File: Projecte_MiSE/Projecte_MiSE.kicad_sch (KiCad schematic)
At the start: 45 parts, among them IC1 MSP430FR2355TPT, J1 C_DFrobot, J10 Conn_GND_TP, J11 Conn_TXD_TP, J12 Conn_RXD_TP, J2 Conn_SWB, J3 ESP01_WIFI, J4 URM10, J5 Conn_GND_TP, J6 Conn_ACLK_TP, J7 Conn_SMCLK_TP, J8 Conn_SDA_TP, J9 Conn_SCL_TP, SW1 ~{RST}, U1 LMV324, Y1 Crystal_GND3

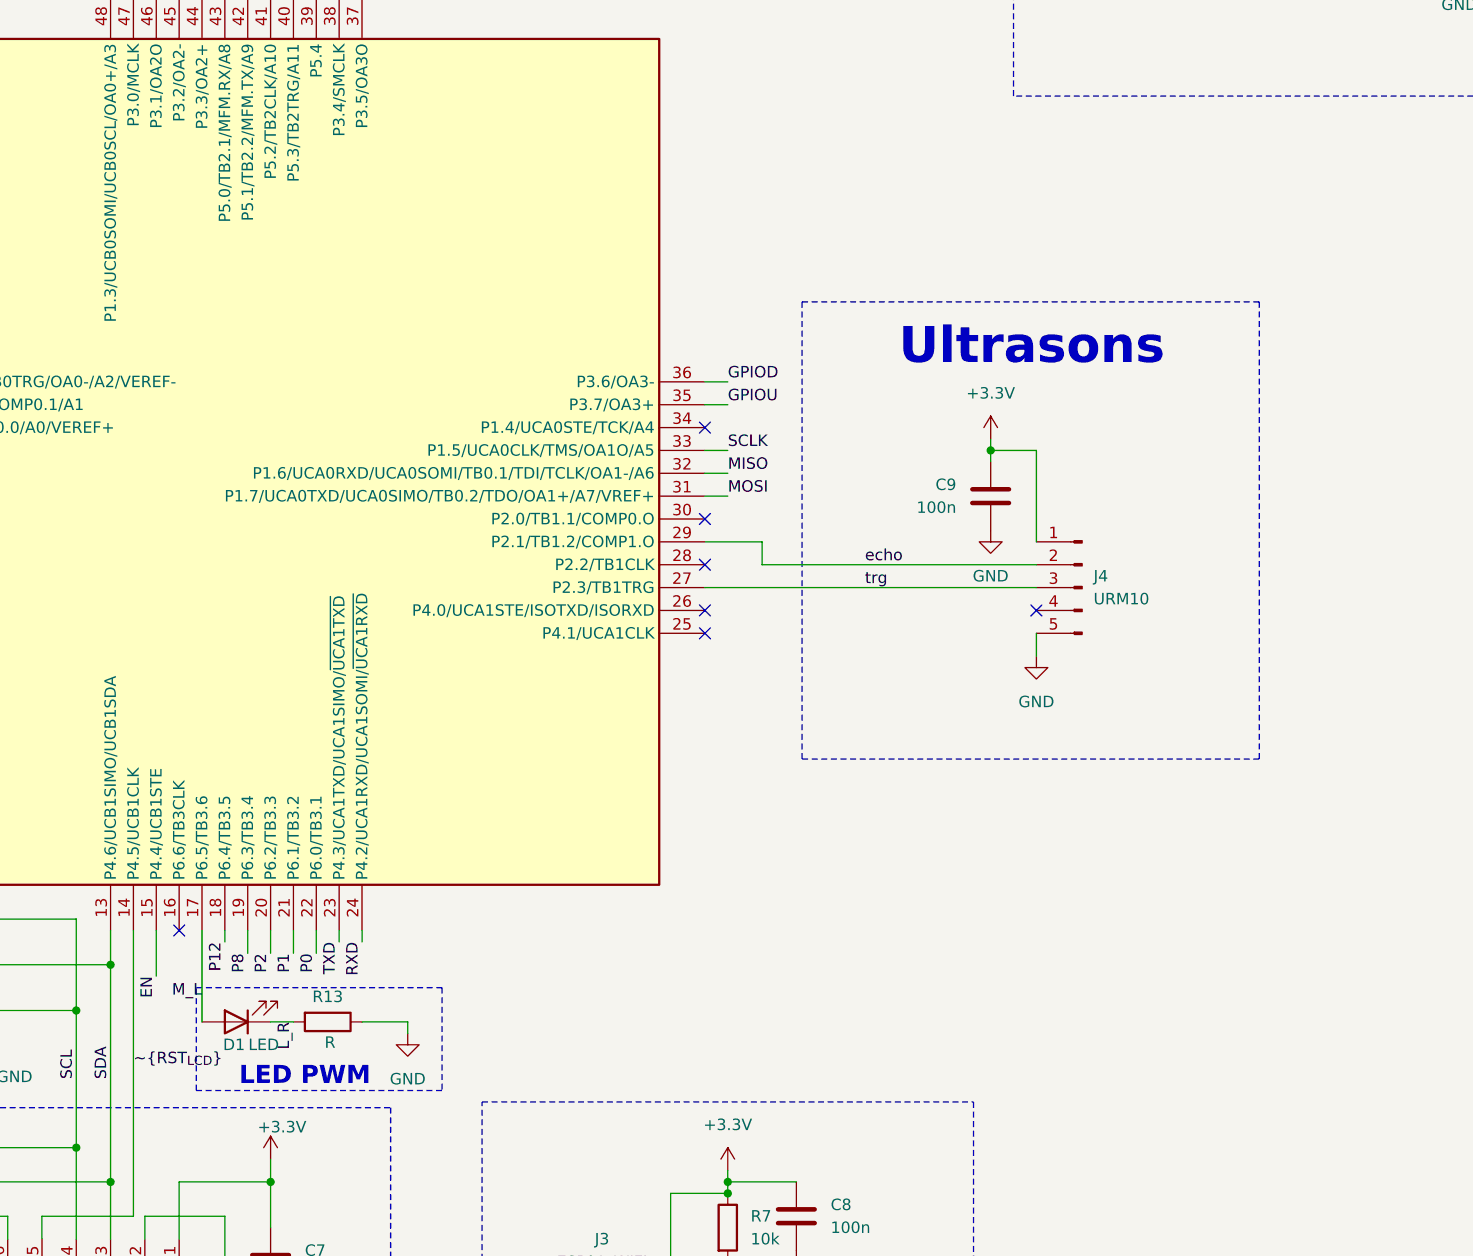
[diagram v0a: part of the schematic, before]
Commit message: footprints and layout
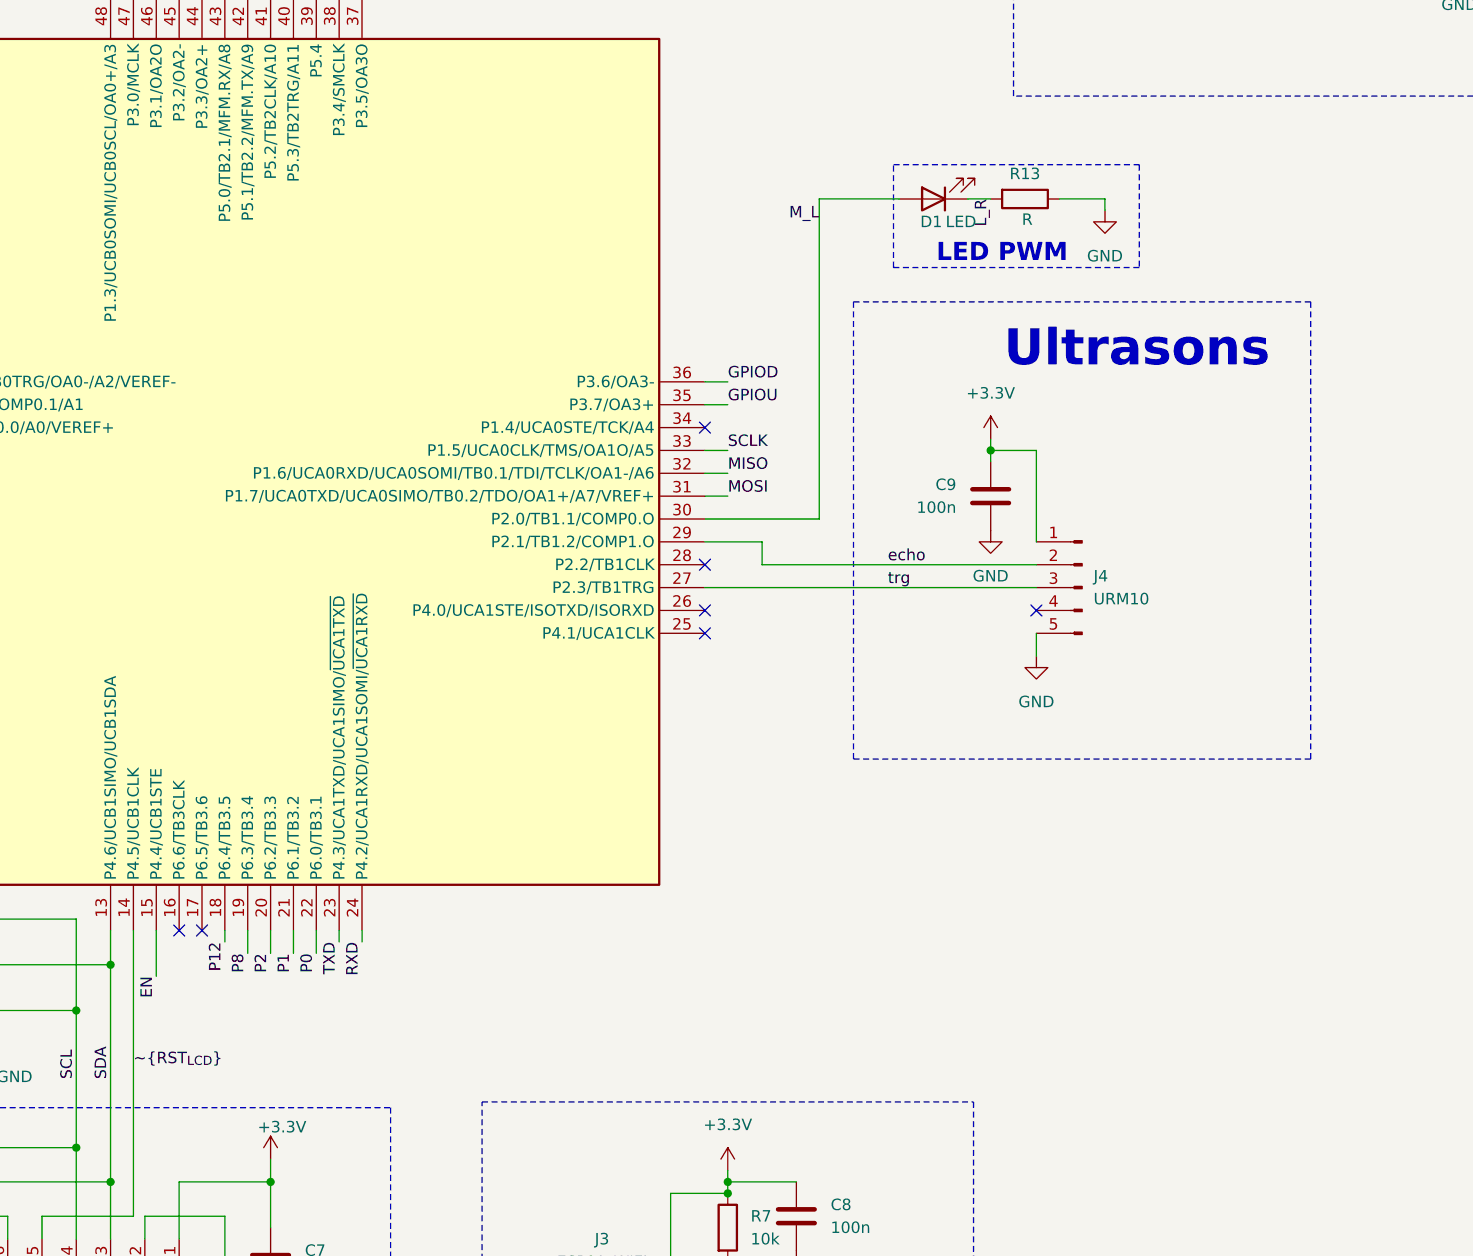
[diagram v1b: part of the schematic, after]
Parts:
- J10, J11, J12, J5, J6, J7, J8, J9: footprint Connector_PinHeader_1.00mm:PinHeader_1x01_P1.00mm_Vertical -> Connector_PinHeader_2.54mm:PinHeader_1x01_P2.54mm_Vertical
- J4: footprint Connector_PinSocket_2.54mm:PinSocket_1x05_P2.54mm_Vertical -> Connector_PinHeader_2.54mm:PinHeader_1x05_P2.54mm_Vertical
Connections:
- net M_L: now also IC1.30 (P2.0/TB1.1/COMP0.O); no longer IC1.17 (P6.5/TB3.6)
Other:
- moved on the sheet: D1, R13
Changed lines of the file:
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@@
 	)
 	(rectangle
-		(start 159.385 215.9)
-		(end 186.69 227.33)
+		(start 236.855 124.46)
+		(end 264.16 135.89)
 		(stroke
 			(width 0)
@@
 	)
 	(rectangle
-		(start 226.695 139.7)
-		(end 277.495 190.5)
+		(start 232.41 139.7)
+		(end 283.21 190.5)
 		(stroke
 			(width 0)
@@
 	(text "Ultrasons\n"
 		(exclude_from_sim no)
-		(at 252.222 144.78 0)
+		(at 263.906 145.034 0)
 		(effects
 			(font
@@
 	(text "LED PWM"
 		(exclude_from_sim no)
-		(at 171.45 225.806 0)
+		(at 248.92 134.366 0)
 		(effects
 			(font
@@
 	)
 	(no_connect
-		(at 215.9 163.83)
-	)
-	(no_connect
 		(at 252.73 173.99)
 	)
@@
 	)
 	(no_connect
+		(at 160.02 209.55)
+	)
+	(no_connect
 		(at 210.82 252.73)
 	)
@@
 	(wire
 		(pts
+			(xy 215.9 163.83) (xy 228.6 163.83)
+		)
+		(stroke
+			(width 0)
+			(type default)
+		)
+	)
+	(wire
+		(pts
 			(xy 66.04 247.65) (xy 69.85 247.65)
 		)
@@
 	(wire
 		(pts
+			(xy 228.6 128.27) (xy 237.49 128.27)
+		)
+		(stroke
+			(width 0)
+			(type default)
+		)
+	)
+	(wire
+		(pts
 			(xy 49.53 149.86) (xy 49.53 151.13)
 		)
@@
 	(wire
 		(pts
+			(xy 228.6 163.83) (xy 228.6 128.27)
+		)
+		(stroke
+			(width 0)
+			(type default)
+		)
+	)
+	(wire
+		(pts
 			(xy 187.96 68.58) (xy 187.96 71.12)
 		)
@@
 	(wire
 		(pts
-			(xy 160.02 209.55) (xy 160.02 219.71)
-		)
-		(stroke
-			(width 0)
-			(type default)
-		)
-	)
-	(wire
-		(pts
 			(xy 317.5 91.44) (xy 317.5 99.06)
 		)
@@
 	(wire
 		(pts
-			(xy 177.8 219.71) (xy 182.88 219.71)
+			(xy 255.27 128.27) (xy 260.35 128.27)
 		)
 		(stroke
@@
 	(wire
 		(pts
-			(xy 167.64 219.71) (xy 170.18 219.71)
+			(xy 245.11 128.27) (xy 247.65 128.27)
 		)
 		(stroke
@@
 	(wire
 		(pts
-			(xy 182.88 219.71) (xy 182.88 220.98)
+			(xy 260.35 128.27) (xy 260.35 129.54)
 		)
 		(stroke
@@
 	)
 	(label "M_L"
-		(at 160.02 217.17 180)
+		(at 228.6 130.81 180)
 		(effects
 			(font
@@
 	)
 	(label "echo"
-		(at 233.68 168.91 0)
+		(at 236.22 168.91 0)
 		(effects
 			(font
@@
 	)
 	(label "trg"
-		(at 233.68 171.45 0)
+		(at 236.22 171.45 0)
 		(effects
 			(font
@@
 	)
 	(label "L_R"
-		(at 170.18 219.71 270)
+		(at 247.65 128.27 270)
 		(effects
 			(font
@@
 			)
 		)
-		(property "Footprint" "Connector_PinHeader_1.00mm:PinHeader_1x01_P1.00mm_Vertical"
+		(property "Footprint" "Connector_PinHeader_2.54mm:PinHeader_1x01_P2.54mm_Vertical"
 			(at 128.27 213.36 0)
 			(effects
@@
 	(symbol
 		(lib_id "power:GND")
-		(at 182.88 220.98 0)
+		(at 260.35 129.54 0)
 		(unit 1)
 		(exclude_from_sim no)
@@
 		(fields_autoplaced yes)
 		(property "Reference" "#PWR025"
-			(at 182.88 227.33 0)
+			(at 260.35 135.89 0)
 			(effects
 				(font
@@
 		)
 		(property "Value" "GND"
-			(at 182.88 226.06 0)
+			(at 260.35 134.62 0)
 			(effects
 				(font
@@
 		)
 		(property "Footprint" ""
-			(at 182.88 220.98 0)
+			(at 260.35 129.54 0)
 			(effects
 				(font
@@
 		)
 		(property "Datasheet" ""
-			(at 182.88 220.98 0)
+			(at 260.35 129.54 0)
 			(effects
 				(font
@@
 		)
 		(property "Description" "Power symbol creates a global label with name \"GND\" , ground"
-			(at 182.88 220.98 0)
+			(at 260.35 129.54 0)
 			(effects
 				(font
@@
 			)
 		)
-		(property "Footprint" "Connector_PinHeader_1.00mm:PinHeader_1x01_P1.00mm_Vertical"
+		(property "Footprint" "Connector_PinHeader_2.54mm:PinHeader_1x01_P2.54mm_Vertical"
 			(at 231.14 252.73 0)
 			(effects
@@
 	(symbol
 		(lib_id "Device:R")
-		(at 173.99 219.71 270)
+		(at 251.46 128.27 270)
 		(unit 1)
 		(exclude_from_sim no)
@@
 		(dnp no)
 		(property "Reference" "R13"
-			(at 173.99 216.916 90)
+			(at 251.46 125.476 90)
 			(effects
 				(font
@@
 		)
 		(property "Value" "R"
-			(at 174.244 221.996 90)
+			(at 251.714 130.556 90)
 			(effects
 				(font
@@
 		)
 		(property "Footprint" "Resistor_SMD:R_0805_2012Metric"
-			(at 173.99 217.932 90)
+			(at 251.46 126.492 90)
 			(effects
 				(font
@@
 		)
 		(property "Datasheet" "~"
-			(at 173.99 219.71 0)
+			(at 251.46 128.27 0)
 			(effects
 				(font
@@
 		)
 		(property "Description" "Resistor"
-			(at 173.99 219.71 0)
+			(at 251.46 128.27 0)
 			(effects
 				(font
@@
 			)
 		)
-		(property "Footprint" "Connector_PinHeader_1.00mm:PinHeader_1x01_P1.00mm_Vertical"
+		(property "Footprint" "Connector_PinHeader_2.54mm:PinHeader_1x01_P2.54mm_Vertical"
 			(at 76.2 105.41 0)
 			(effects
@@
 			)
 		)
-		(property "Footprint" "Connector_PinHeader_1.00mm:PinHeader_1x01_P1.00mm_Vertical"
+		(property "Footprint" "Connector_PinHeader_2.54mm:PinHeader_1x01_P2.54mm_Vertical"
 			(at 74.93 111.76 0)
 			(effects
@@
 			)
 		)
-		(property "Footprint" "Connector_PinHeader_1.00mm:PinHeader_1x01_P1.00mm_Vertical"
+		(property "Footprint" "Connector_PinHeader_2.54mm:PinHeader_1x01_P2.54mm_Vertical"
 			(at 128.27 218.44 0)
 			(effects
@@
 			)
 		)
-		(property "Footprint" "Connector_PinHeader_1.00mm:PinHeader_1x01_P1.00mm_Vertical"
+		(property "Footprint" "Connector_PinHeader_2.54mm:PinHeader_1x01_P2.54mm_Vertical"
 			(at 128.27 224.79 0)
 			(effects
@@
 			)
 		)
-		(property "Footprint" "Connector_PinHeader_1.00mm:PinHeader_1x01_P1.00mm_Vertical"
+		(property "Footprint" "Connector_PinHeader_2.54mm:PinHeader_1x01_P2.54mm_Vertical"
 			(at 76.2 100.33 0)
 			(effects
@@
 			)
 		)
-		(property "Footprint" "Connector_PinHeader_1.00mm:PinHeader_1x01_P1.00mm_Vertical"
+		(property "Footprint" "Connector_PinHeader_2.54mm:PinHeader_1x01_P2.54mm_Vertical"
 			(at 229.87 257.81 0)
 			(effects
@@
 	(symbol
 		(lib_id "Device:LED")
-		(at 163.83 219.71 180)
+		(at 241.3 128.27 180)
 		(unit 1)
 		(exclude_from_sim no)
@@
 		(dnp no)
 		(property "Reference" "D1"
-			(at 163.576 222.25 0)
+			(at 241.046 130.81 0)
 			(effects
 				(font
@@
 		)
 		(property "Value" "LED"
-			(at 166.878 222.25 0)
+			(at 244.348 130.81 0)
 			(effects
 				(font
@@
 		)
 		(property "Footprint" "LED_SMD:LED_0805_2012Metric"
-			(at 163.83 219.71 0)
+			(at 241.3 128.27 0)
 			(effects
 				(font
@@
 		)
 		(property "Datasheet" "~"
-			(at 163.83 219.71 0)
+			(at 241.3 128.27 0)
 			(effects
 				(font
@@
 		)
 		(property "Description" "Light emitting diode"
-			(at 163.83 219.71 0)
+			(at 241.3 128.27 0)
 			(effects
 				(font
@@
 			)
 		)
-		(property "Footprint" "Connector_PinSocket_2.54mm:PinSocket_1x05_P2.54mm_Vertical"
+		(property "Footprint" "Connector_PinHeader_2.54mm:PinHeader_1x05_P2.54mm_Vertical"
 			(at 257.81 171.45 0)
 			(effects
